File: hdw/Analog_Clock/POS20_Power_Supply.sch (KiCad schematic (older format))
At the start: 31 parts

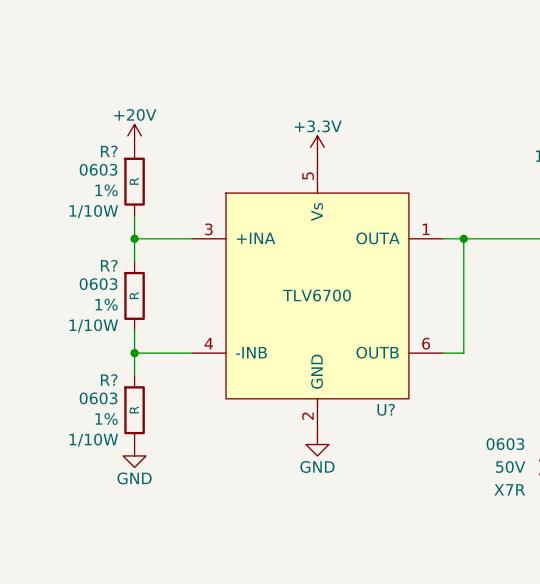
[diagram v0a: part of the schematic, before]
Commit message: more analog work, added some more sch stuff
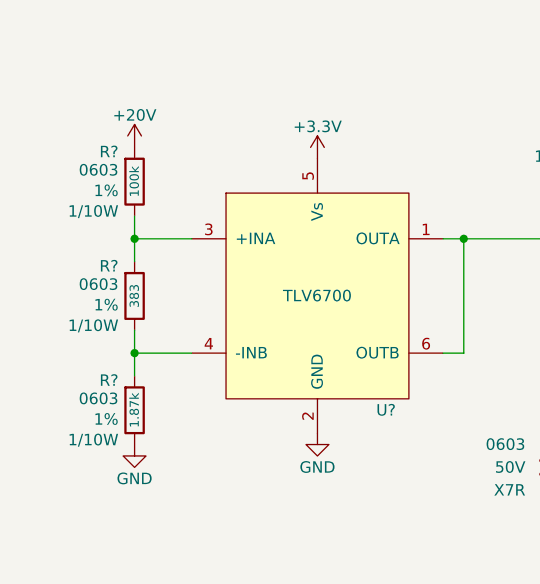
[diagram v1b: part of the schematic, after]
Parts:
- R?: value R -> 1.87k
- R?: value R -> 383
- R?: value R -> 100k
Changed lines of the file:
@@
 $Descr A 11000 8500
 encoding utf-8
-Sheet 6 23
+Sheet 6 24
 Title "VFD Clock"
 Date "2019-04-11"
@@
 P 2050 7100
 F 0 "R?" H 2120 7230 50  0000 L CNN
-F 1 "R" V 2050 7100 40  0000 C CNN
+F 1 "1.87k" V 2050 7100 40  0000 C CNN
 F 2 "Resistors_SMD:R_0603" H 2050 7100 50  0001 C CNN
 F 3 "" H 2050 7100 50  0001 C CNN
@@
 P 2050 6600
 F 0 "R?" H 2120 6730 50  0000 L CNN
-F 1 "R" V 2050 6600 40  0000 C CNN
+F 1 "383" V 2050 6600 40  0000 C CNN
 F 2 "Resistors_SMD:R_0603" H 2050 6600 50  0001 C CNN
 F 3 "" H 2050 6600 50  0001 C CNN
@@
 P 2050 6100
 F 0 "R?" H 2120 6230 50  0000 L CNN
-F 1 "R" V 2050 6100 40  0000 C CNN
+F 1 "100k" V 2050 6100 40  0000 C CNN
 F 2 "Resistors_SMD:R_0603" H 2050 6100 50  0001 C CNN
 F 3 "" H 2050 6100 50  0001 C CNN
@@
 AR Path="/5EAE2D8A/5F3155DF" Ref="R?"  Part="1"
 AR Path="/5E939D31/5F3155DF" Ref="R?"  Part="1"
+AR Path="/5E939D51/5F3155DF" Ref="R?"  Part="1"
 F 0 "R?" V 4850 2340 50  0000 C CNN
 F 1 "10" V 4950 2340 50  0000 C CNN
